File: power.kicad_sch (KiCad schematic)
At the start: 18 parts, among them J1 12402012E212A, J13 Conn_01x02, SW2 SW_SPDT, U3 AP2112K-3.3

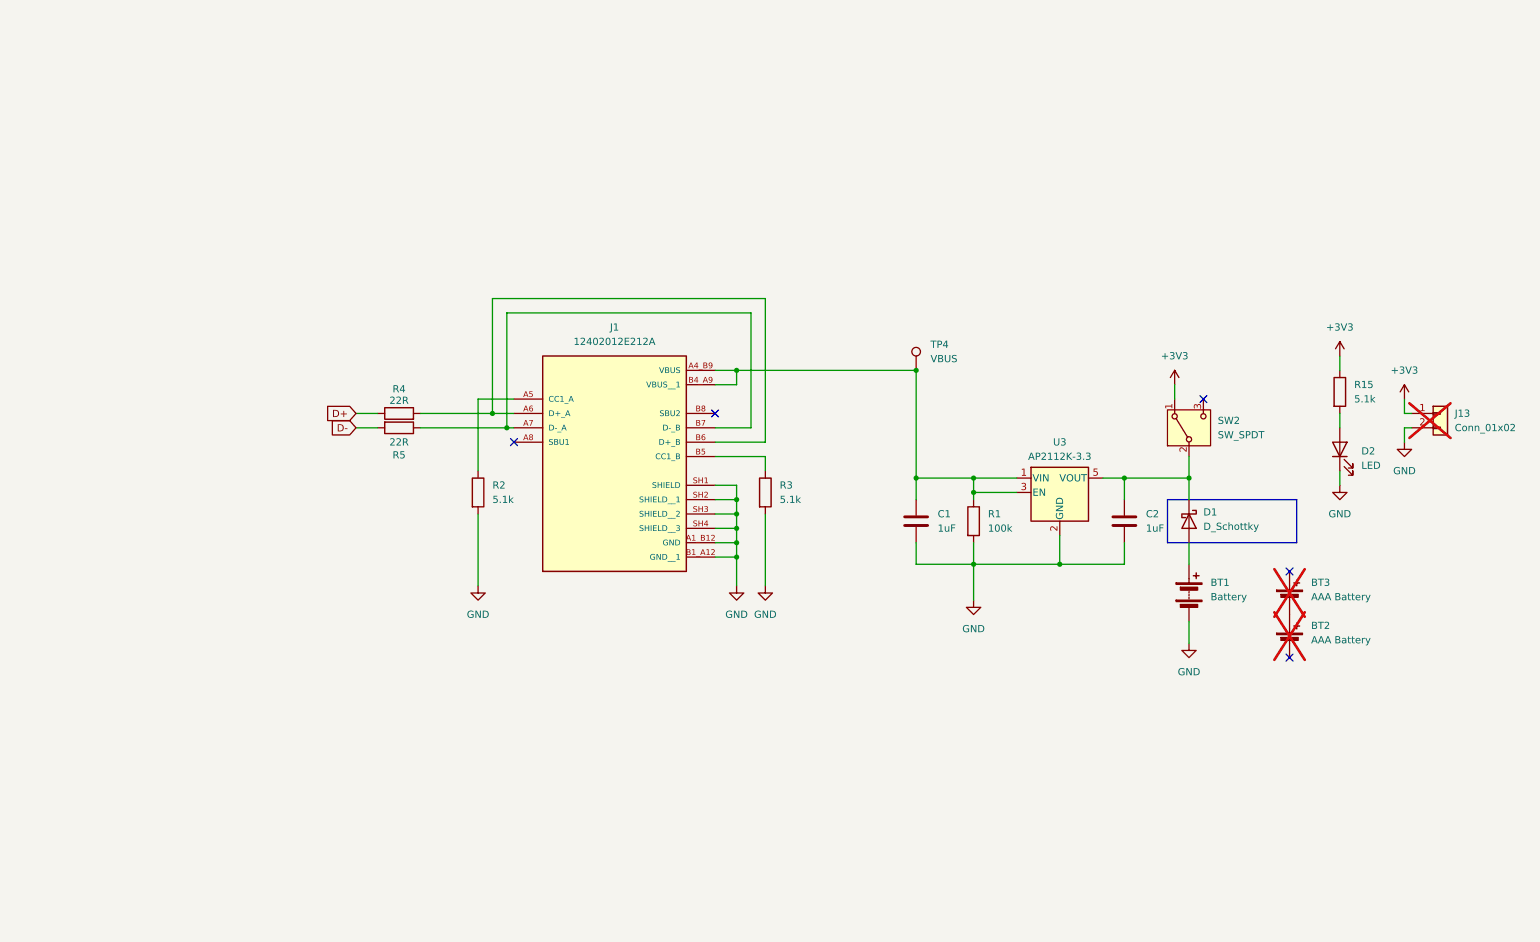
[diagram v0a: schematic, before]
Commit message: Board V3
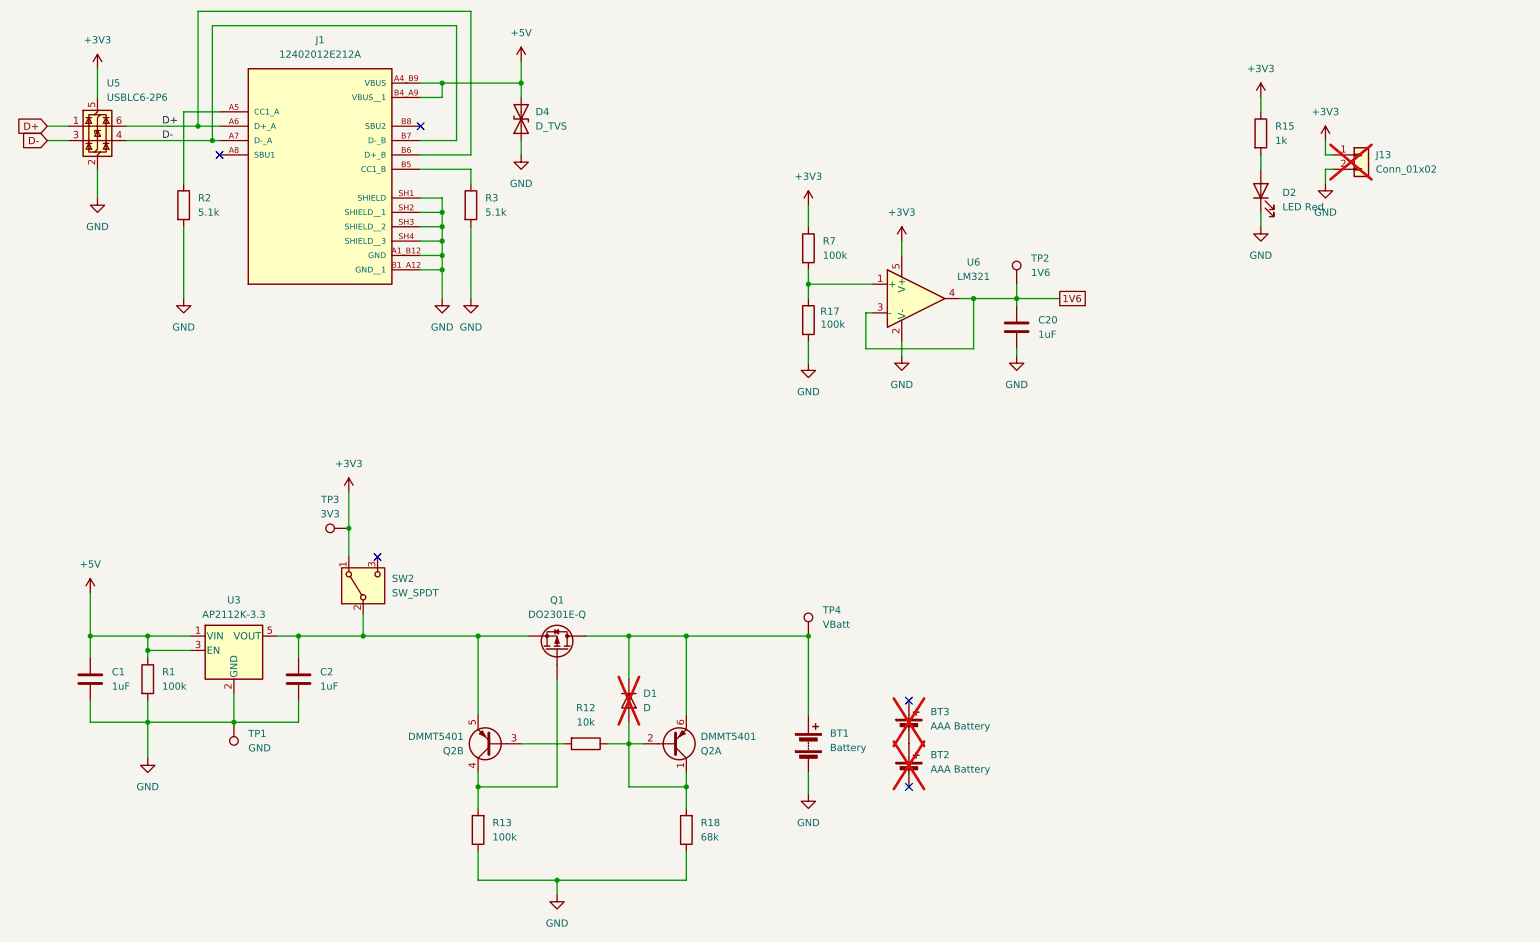
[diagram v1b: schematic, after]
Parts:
- removed D1: D_Schottky, Diode_SMD:D_SOD-123, symbol Device:D_Schottky
- removed R4, R5: 22R, Resistor_SMD:R_0402_1005Metric, symbol Device:R
- added C20: 1uF, Capacitor_SMD:C_0402_1005Metric, symbol Device:C
- added D1: D, Diode_SMD:D_0402_1005Metric, symbol Device:D
- added D4: D_TVS, KUU:SOD-882, symbol Device:D_TVS
- added Q1: DO2301E-Q, Package_TO_SOT_SMD:SOT-23, symbol Device:Q_PMOS
- added Q2: DMMT5401, Package_TO_SOT_SMD:SOT-23-6, symbol Transistor_BJT:DMMT5401
- added R12: 10k, Resistor_SMD:R_0402_1005Metric, symbol Device:R
- added R13, R17, R7: 100k, Resistor_SMD:R_0402_1005Metric, symbol Device:R
- added R18: 68k, Resistor_SMD:R_0402_1005Metric, symbol Device:R
- added TP1: GND, TestPoint:TestPoint_Pad_1.0x1.0mm, symbol Connector:TestPoint
- added TP2: 1V6, TestPoint:TestPoint_Pad_1.0x1.0mm, symbol Connector:TestPoint
- added TP3: 3V3, TestPoint:TestPoint_Pad_1.0x1.0mm, symbol Connector:TestPoint
- added U5: USBLC6-2P6, Package_TO_SOT_SMD:SOT-666, symbol Power_Protection:USBLC6-2P6
- added U6: LM321, Package_TO_SOT_SMD:SOT-23-5, symbol Amplifier_Operational:LM321
- BT1: footprint Battery:BatteryHolder_Keystone_2468_2xAAA -> battery:BatteryHolder_Keystone_2468_2xAAA; Alibaba (none) -> https://www.alibaba.com/product-detail/BH2AAATH-2-AAA-Batte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; Est Cost (1000) (none) -> 0.1959; Height (none) -> 13mm; Manufacturer (none) -> Jinbeili; Part No (none) -> BH2AAATH; Type (none) -> Through Hole
- C1: Est Cost (1000) (none) -> 0.001; LCSC (none) -> https://www.lcsc.com/product-detail/C7503520.html; Manufacturer (none) -> HRE; Part No (none) -> CGA0402X5R105K100GT; Type (none) -> SMD; Vendor https://www.lcsc.com/product-detail/C6119818.html -> (none)
- C2: Est Cost 0.0027 -> (none); Est Cost (1000) (none) -> 0.001; LCSC (none) -> https://www.lcsc.com/product-detail/C7503520.html; Manufacturer (none) -> HRE; Part No (none) -> CGA0402X5R105K100GT; Type (none) -> SMD; Vendor https://www.lcsc.com/product-detail/C6119818.html -> (none)
- D2: value LED -> LED Red; Est Cost 0.0022 -> (none); Est Cost (1000) (none) -> 0.0027; LCSC (none) -> https://www.lcsc.com/product-detail/C965799.html; Manufacturer (none) -> XINGLIGHT; Part No (none) -> XL-1608SURC-06; Type (none) -> SMD; Vendor https://www.lcsc.com/product-detail/C965799.html -> (none)
- J1: Est Cost 0.0488 -> (none); Est Cost (1000) (none) -> 0.0497; Height (none) -> 3.26mm; LCSC (none) -> https://www.lcsc.com/product-detail/C2988369.html; Manufacturer (none) -> G-Switch; Part No (none) -> GT-USB-7010ASV; Type (none) -> SMD; Vendor https://www.lcsc.com/product-detail/C2988369.html -> (none)
- R1: Est Cost 0.0007 -> (none); Est Cost (1000) (none) -> 0.0003; LCSC (none) -> https://www.lcsc.com/product-detail/C2906883.html; Manufacturer (none) -> FOJAN; Part No (none) -> FRC0402J104 TS; Type (none) -> SMD; Vendor https://www.lcsc.com/product-detail/C3017691.html -> (none)
- R15: value 5.1k -> 1k; Est Cost 0.0006 -> (none); Est Cost (1000) (none) -> 0.0003; LCSC (none) -> https://www.lcsc.com/product-detail/C3017479.html; Manufacturer (none) -> VO; Part No (none) -> SCR0402J1K; Type (none) -> SMD; Vendor https://www.lcsc.com/product-detail/C49254213.html -> (none)
- R2, R3: Est Cost 0.0006 -> (none); Est Cost (1000) (none) -> 0.0003; LCSC (none) -> https://www.lcsc.com/product-detail/C2906948.html; Manufacturer (none) -> FOJAN; Part No (none) -> FRC0402J512 TS; Type (none) -> SMD; Vendor https://www.lcsc.com/product-detail/C49254213.html -> (none)
- SW2: Est Cost 0.0163 -> (none); Est Cost (1000) (none) -> 0.0163; Height (none) -> 4.4mm; LCSC (none) -> https://www.lcsc.com/product-detail/C431547.html; Manufacturer (none) -> SHOU HAN; Part No (none) -> SK12D07VG3; Type (none) -> SMD; Vendor https://www.lcsc.com/product-detail/C431547.html -> (none)
- TP4: value VBUS -> VBatt; footprint TestPoint:TestPoint_Pad_D1.5mm -> TestPoint:TestPoint_Pad_1.0x1.0mm; now left out of the parts list
- U3: Est Cost 0.062 -> (none); Est Cost (1000) (none) -> 0.0574; Height (none) -> 1.25mm; LCSC (none) -> https://www.lcsc.com/product-detail/C23380830.html?s_z=n_AP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; Manufacturer (none) -> TECH PUBLIC; Part No (none) -> AP2112K-3.3TRG1; Type (none) -> SMD; Vendor https://www.lcsc.com/product-detail/C23380830.html?s_z=n_AP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 -> (none)
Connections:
- net +3V3: now also R7.1, TP3.1, U5.5 (VBUS), U6.5 (V+)
- net D+: now also J1.A6 (D+_A), J1.B6 (D+_B), U5.1 (I/O1), U5.6 (I/O1)
- net D-: now also J1.A7 (D-_A), J1.B7 (D-_B), U5.3 (I/O2), U5.4 (I/O2)
- net GND: now also C20.2, D4.1 (A1), R13.1, R17.2, R18.1, TP1.1, U5.2 (GND), U6.2 (V-)
- net +5V: now reaches C1.1, J1.A4_B9 (VBUS), J1.B4_A9 (VBUS__1), R1.1, U3.1 (VIN), U3.3 (EN)
- net +5V: now also D4.2 (A2); no longer TP4.1
- net at C2.1, SW2.2 (B), U3.5 (VOUT): now also Q1.2 (S), Q2.5 (E2)
- net at BT1.1 (+): now also TP4.1, D1.1 (K), Q1.3 (D), Q2.6 (E1)
- new net: D1.2 (A), Q2.1 (C1), Q2.2 (B1), R12.1, R18.2
- new net: Q2.3 (B2), R12.2
- new net: Q1.1 (G), Q2.4 (C2), R13.2
- new net: R17.1, R7.2, U6.1 (+)
- new net 1V6: C20.1, TP2.1, U6.3 (-), U6.4
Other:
- moved on the sheet: BT1, BT2, BT3, C1, C2, D2, J1, J13, R1, R15, R2, R3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
